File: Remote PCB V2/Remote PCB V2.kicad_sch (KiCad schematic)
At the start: 14 parts, among them SW1 SW_Push, SW2 SW_Push, SW3 SW_Push, SW4 SW_Push, SW5 SW_Push

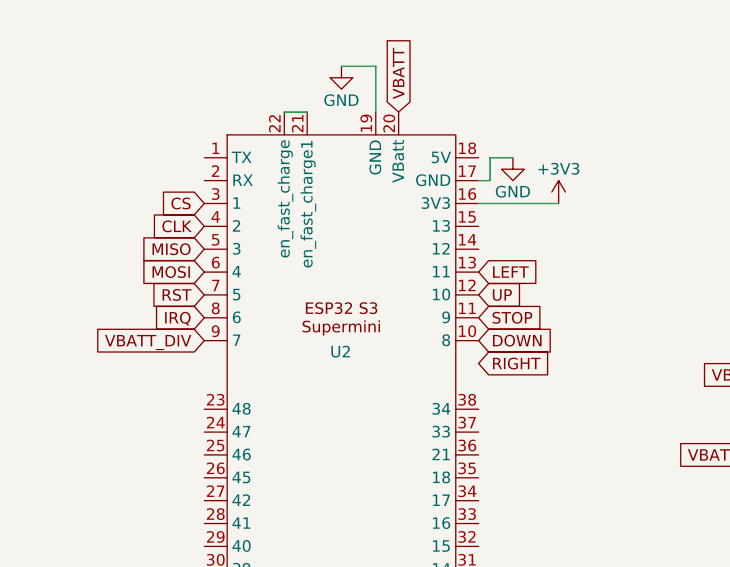
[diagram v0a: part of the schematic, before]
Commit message: V3
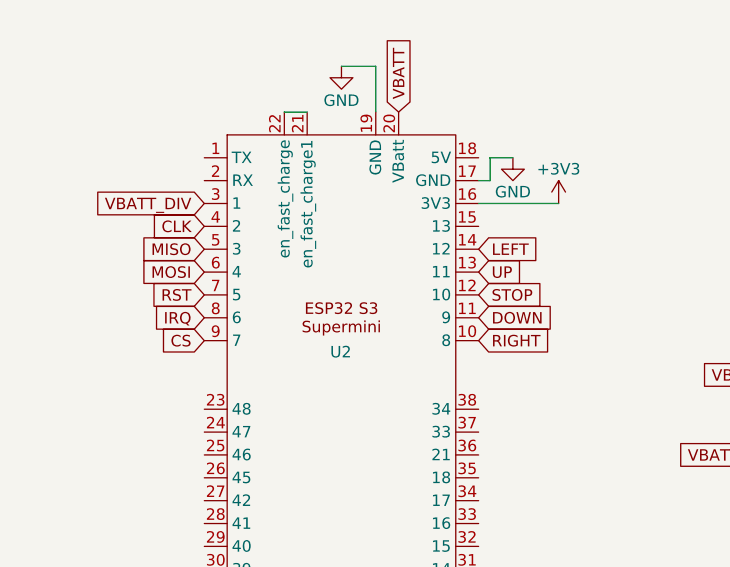
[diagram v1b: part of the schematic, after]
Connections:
- net CS: now also U2.9 (7); no longer U2.3 (1)
- net DOWN: now also U2.11 (9); no longer U2.10 (8)
- net LEFT: now also U2.14 (12); no longer U2.13 (11)
- net RIGHT: now also U2.10 (8)
- net STOP: now also U2.12 (10); no longer U2.11 (9)
- net UP: now also U2.13 (11); no longer U2.12 (10)
- net VBATT_DIV: now also U2.3 (1); no longer U2.9 (7)
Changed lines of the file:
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@@
     )
   )
-  (global_label "LEFT" (shape input) (at 118.11 120.65 0) (fields_autoplaced)
+  (global_label "RIGHT" (shape input) (at 118.11 128.27 0) (fields_autoplaced)
     (effects (font (size 1.27 1.27)) (justify left))
-    (property "Intersheetrefs" "${INTERSHEET_REFS}" (at 125.3285 120.65 0)
+    (property "Intersheetrefs" "${INTERSHEET_REFS}" (at 126.5381 128.27 0)
       (effects (font (size 1.27 1.27)) (justify left) hide)
     )
@@
     )
   )
-  (global_label "UP" (shape input) (at 118.11 123.19 0) (fields_autoplaced)
-    (effects (font (size 1.27 1.27)) (justify left))
-    (property "Intersheetrefs" "${INTERSHEET_REFS}" (at 123.6957 123.19 0)
-      (effects (font (size 1.27 1.27)) (justify left) hide)
-    )
-  )
   (global_label "STOP" (shape input) (at 85.09 78.74 180) (fields_autoplaced)
     (effects (font (size 1.27 1.27)) (justify right))
     (property "Intersheetrefs" "${INTERSHEET_REFS}" (at 77.3272 78.74 0)
       (effects (font (size 1.27 1.27)) (justify right) hide)
-    )
-  )
-  (global_label "STOP" (shape input) (at 118.11 125.73 0) (fields_autoplaced)
-    (effects (font (size 1.27 1.27)) (justify left))
-    (property "Intersheetrefs" "${INTERSHEET_REFS}" (at 125.8728 125.73 0)
-      (effects (font (size 1.27 1.27)) (justify left) hide)
     )
   )
@@
     )
   )
-  (global_label "VBATT_DIV" (shape input) (at 87.63 128.27 180) (fields_autoplaced)
-    (effects (font (size 1.27 1.27)) (justify right))
-    (property "Intersheetrefs" "${INTERSHEET_REFS}" (at 75.3314 128.27 0)
-      (effects (font (size 1.27 1.27)) (justify right) hide)
+  (global_label "STOP" (shape input) (at 118.11 123.19 0) (fields_autoplaced)
+    (effects (font (size 1.27 1.27)) (justify left))
+    (property "Intersheetrefs" "${INTERSHEET_REFS}" (at 125.8728 123.19 0)
+      (effects (font (size 1.27 1.27)) (justify left) hide)
     )
   )
@@
     )
   )
-  (global_label "DOWN" (shape input) (at 118.11 128.27 0) (fields_autoplaced)
-    (effects (font (size 1.27 1.27)) (justify left))
-    (property "Intersheetrefs" "${INTERSHEET_REFS}" (at 126.4776 128.27 0)
-      (effects (font (size 1.27 1.27)) (justify left) hide)
+  (global_label "VBATT_DIV" (shape input) (at 87.63 113.03 180) (fields_autoplaced)
+    (effects (font (size 1.27 1.27)) (justify right))
+    (property "Intersheetrefs" "${INTERSHEET_REFS}" (at 75.3314 113.03 0)
+      (effects (font (size 1.27 1.27)) (justify right) hide)
     )
   )
@@
     (property "Intersheetrefs" "${INTERSHEET_REFS}" (at 203.1614 52.07 0)
       (effects (font (size 1.27 1.27)) (justify left) hide)
-    )
-  )
-  (global_label "CS" (shape input) (at 87.63 113.03 180) (fields_autoplaced)
-    (effects (font (size 1.27 1.27)) (justify right))
-    (property "Intersheetrefs" "${INTERSHEET_REFS}" (at 82.1653 113.03 0)
-      (effects (font (size 1.27 1.27)) (justify right) hide)
     )
   )
@@
     )
   )
+  (global_label "LEFT" (shape input) (at 118.11 118.11 0) (fields_autoplaced)
+    (effects (font (size 1.27 1.27)) (justify left))
+    (property "Intersheetrefs" "${INTERSHEET_REFS}" (at 125.3285 118.11 0)
+      (effects (font (size 1.27 1.27)) (justify left) hide)
+    )
+  )
   (global_label "LEFT" (shape input) (at 74.93 69.85 180) (fields_autoplaced)
     (effects (font (size 1.27 1.27)) (justify right))
     (property "Intersheetrefs" "${INTERSHEET_REFS}" (at 67.7115 69.85 0)
       (effects (font (size 1.27 1.27)) (justify right) hide)
+    )
+  )
+  (global_label "DOWN" (shape input) (at 118.11 125.73 0) (fields_autoplaced)
+    (effects (font (size 1.27 1.27)) (justify left))
+    (property "Intersheetrefs" "${INTERSHEET_REFS}" (at 126.4776 125.73 0)
+      (effects (font (size 1.27 1.27)) (justify left) hide)
     )
   )
@@
     )
   )
-  (global_label "RIGHT" (shape input) (at 118.11 130.81 0) (fields_autoplaced)
+  (global_label "UP" (shape input) (at 118.11 120.65 0) (fields_autoplaced)
     (effects (font (size 1.27 1.27)) (justify left))
-    (property "Intersheetrefs" "${INTERSHEET_REFS}" (at 126.5381 130.81 0)
+    (property "Intersheetrefs" "${INTERSHEET_REFS}" (at 123.6957 120.65 0)
       (effects (font (size 1.27 1.27)) (justify left) hide)
     )
@@
       (effects (font (size 1.27 1.27)) (justify right) hide)
     )
+  )
+  (global_label "CS" (shape input) (at 87.63 128.27 180) (fields_autoplaced)
+    (effects (font (size 1.27 1.27)) (justify right))
+    (property "Intersheetrefs" "${INTERSHEET_REFS}" (at 82.1653 128.27 0)
+      (effects (font (size 1.27 1.27)) (justify right) hide)
+    )
